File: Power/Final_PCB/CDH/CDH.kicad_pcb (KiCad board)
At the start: 2 copper layers, 85 x 85 mm, 22 parts, among them IC1 TEENSY_4.1, J1 Left_Header, J2 Right_Header, J3 Transceiver header, U3 DPS310XTSA1, U4 HTS221

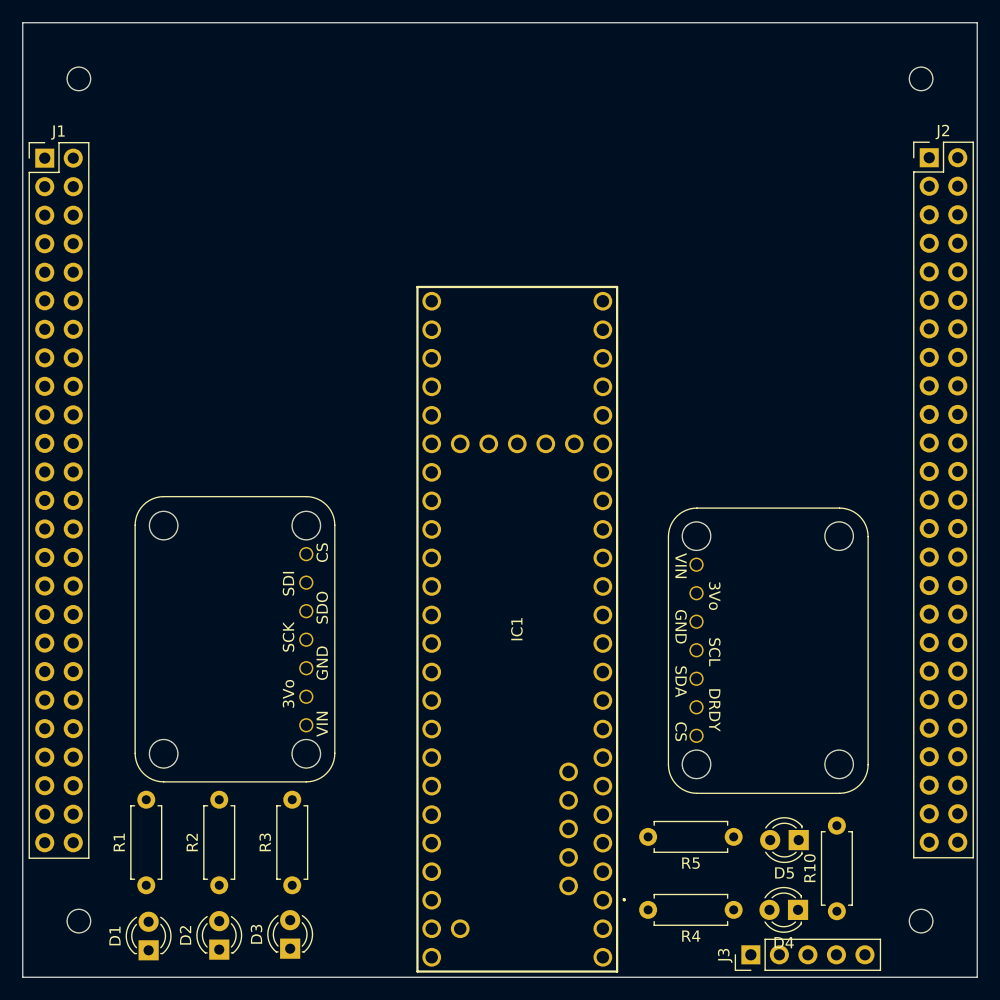
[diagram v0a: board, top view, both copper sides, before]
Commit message: Completed CDH Board
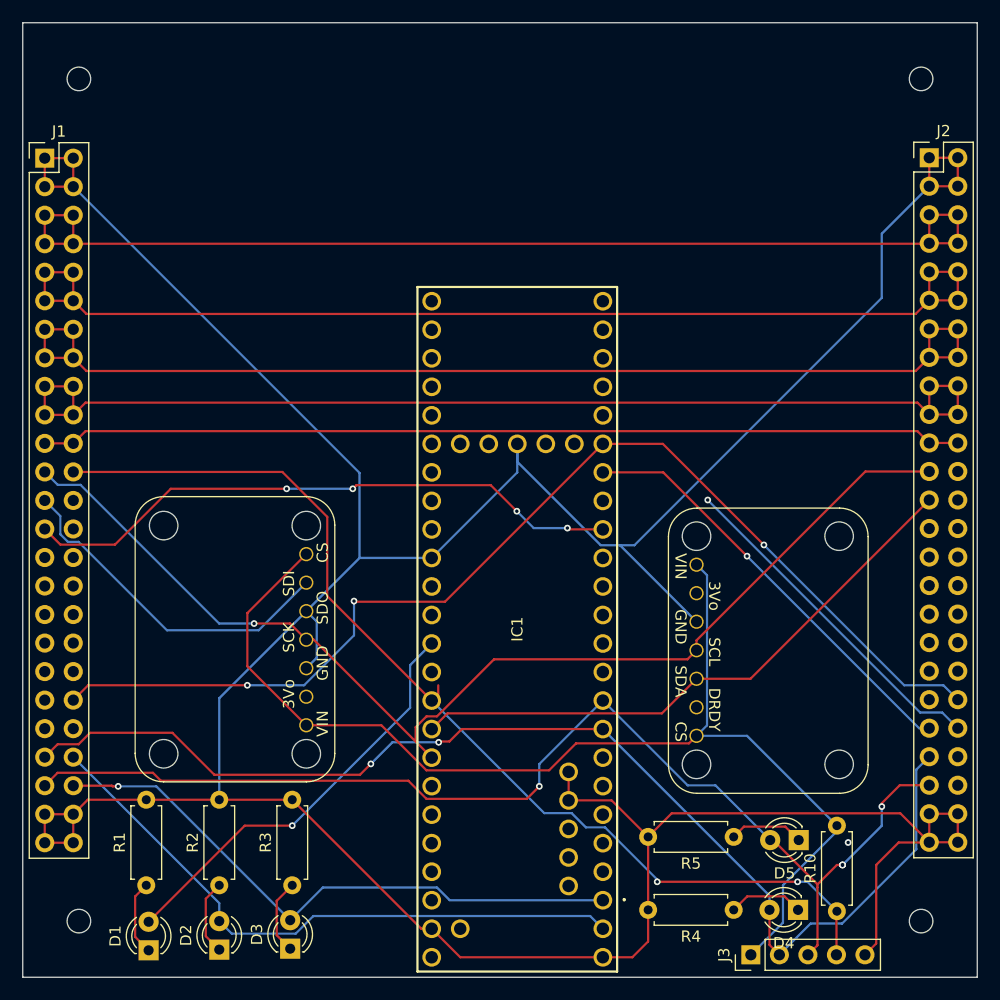
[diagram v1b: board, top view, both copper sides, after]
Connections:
- IC1 pad 14: L298N_1_ENA -> unconnected-(IC1-A0-Pad14)
- IC1 pad 20: L298N_1_IN2 -> unconnected-(IC1-A6-Pad20)
- IC1 pad 21: L298N_1_IN1 -> unconnected-(IC1-A7-Pad21)
- IC1 pad 34: L298N_2_IN1 -> unconnected-(IC1-RX8-Pad34)
- IC1 pad 35: L298N_2_IN2 -> unconnected-(IC1-TX8-Pad35)
- IC1 pad 36: L298N_1_IN3 -> unconnected-(IC1-CS_2-Pad36)
- IC1 pad 37: L298N_1_IN4 -> unconnected-(IC1-CS_3-Pad37)
- IC1 pad 38: L298N_2_ENA -> unconnected-(IC1-A14-Pad38)
- IC1 pad 39: L298N_1_ENB -> unconnected-(IC1-A15-Pad39)
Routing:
- net GND: track 0.00 -> 323.5 mm
- net SDA: track 0.00 -> 143.2 mm
- net XB_RESET: track 0.00 -> 139.4 mm, vias 0 -> 3
- net RX2: track 0.00 -> 105.3 mm, vias 0 -> 2
- net +3V3: track 0.00 -> 103.8 mm
- net TX2: track 0.00 -> 103.2 mm, vias 0 -> 4
- net SCL: track 0.00 -> 102.0 mm, vias 0 -> 1
- net GNSS_PPS: track 0.00 -> 99.5 mm, vias 0 -> 3
- net GNSS_FIX: track 0.00 -> 97.7 mm, vias 0 -> 1
- net 14.8V: track 0.00 -> 97.5 mm
- net 5V: track 0.00 -> 97.5 mm
- net 28V: track 0.00 -> 97.4 mm
- net TX1: track 0.00 -> 97.0 mm, vias 0 -> 1
- net 3V3: track 0.00 -> 96.6 mm
- net GNSS_EN: track 0.00 -> 95.6 mm, vias 0 -> 1
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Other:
- copper layers 2 -> 4

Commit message: Finalising Sensors Schematic
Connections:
- IC1 pad 2: unconnected-(IC1-OUT2-Pad2) -> BNO_INT
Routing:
- net BNO_INT: track 81.8 -> 138.8 mm
